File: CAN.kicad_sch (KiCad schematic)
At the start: 10 parts, among them J5 Conn_01x02_Pin, U5 TCAN337, U6 CDSOT23-T24CAN

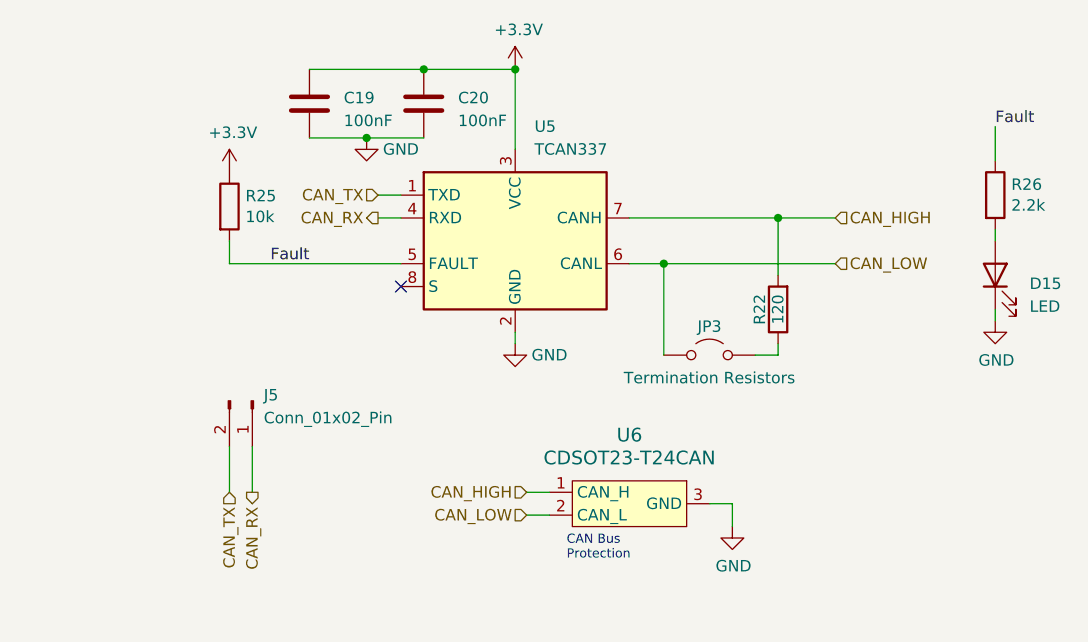
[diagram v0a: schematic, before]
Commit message: finished? power on sch
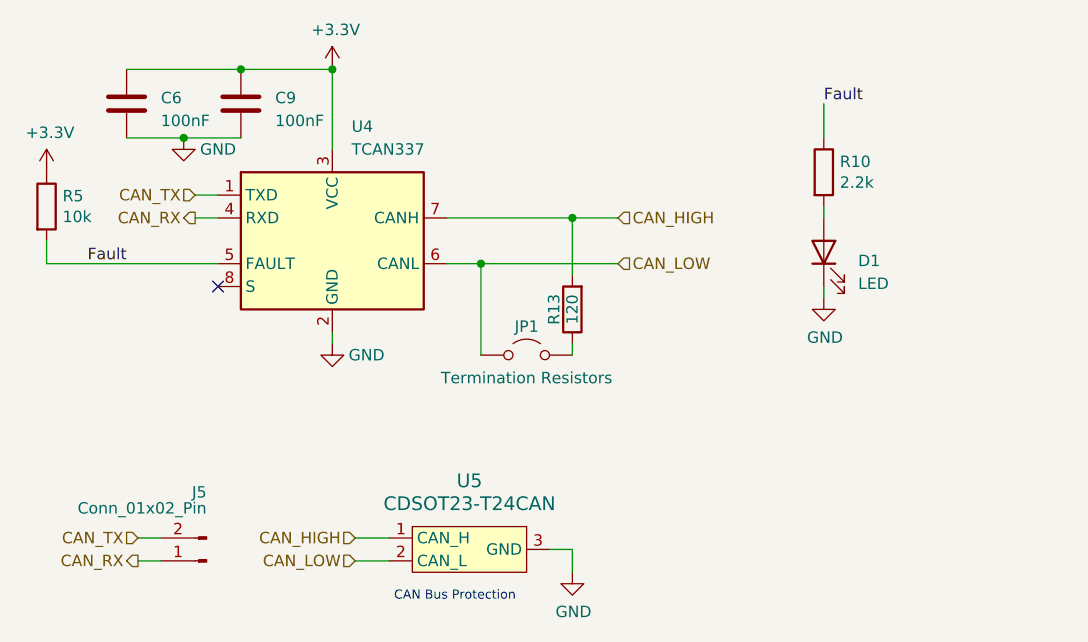
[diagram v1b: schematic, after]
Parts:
- renumbered C19 to C6, C20 to C9, D15 to D1, JP3 to JP1, R26 to R10, R22 to R13, R25 to R5, U5 to U4, U6 to U5
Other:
- moved on the sheet: C6, C9, D1, J5, JP1, R10, R13, R5, U4, U5
